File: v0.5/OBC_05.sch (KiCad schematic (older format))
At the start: 0 parts

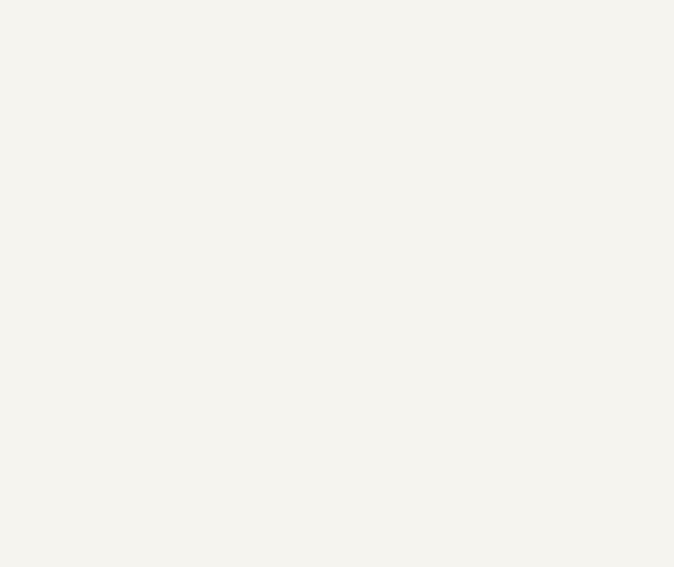
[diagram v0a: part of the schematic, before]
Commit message: Updated power setup
We now either go over USB_5V or through the 104 connector. For flexibility, our own 3V3 header is included, but this is identical to the 104 connector one.
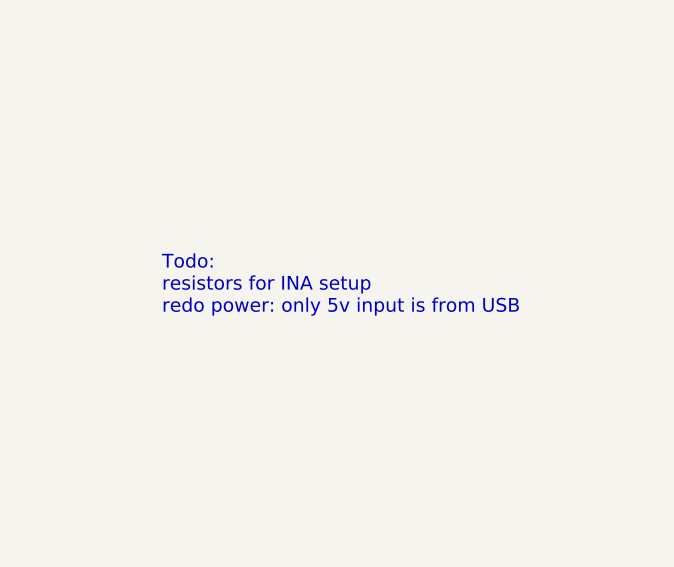
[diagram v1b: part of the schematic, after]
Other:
- note added: "Todo:\nresistors for INA setup\nredo power: only 5v input is from USB"
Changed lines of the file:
@@
 F1 "Extra.sch" 60
 $EndSheet
+Text Notes 5200 3250 0    60   ~ 0
+Todo:\nresistors for INA setup\nredo power: only 5v input is from USB
 $EndSCHEMATC

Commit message: Routed the nasty stuff
Needs cleanup but the 104 connector is almost done
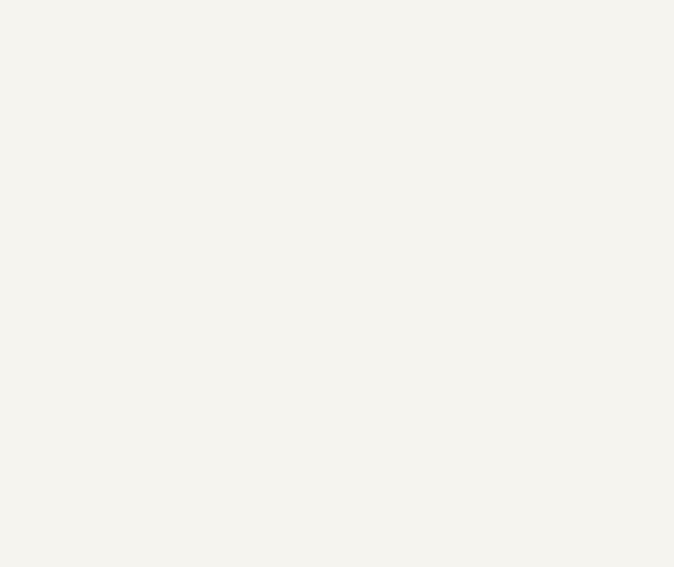
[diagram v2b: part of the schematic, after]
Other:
- note removed: "Todo:\nresistors for INA setup\nredo power: only 5v input is from USB"
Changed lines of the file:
@@
 F1 "Extra.sch" 60
 $EndSheet
-Text Notes 5200 3250 0    60   ~ 0
-Todo:\nresistors for INA setup\nredo power: only 5v input is from USB
 $EndSCHEMATC
